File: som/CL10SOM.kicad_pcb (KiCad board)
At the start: 4 copper layers, 34.9 x 31.9 mm, 53 parts, among them IC1 10CL025YU256C8G, J1 Conn_01x02_Pin, U1 MT46H32M16LFBF-5 IT:C, U2 MX25L12833FM2, U6 AT93C46DN-SH-T, U7 SG3225CAN 50.0000M-TJGA6, X1 DF40C-120DS-0.4V51

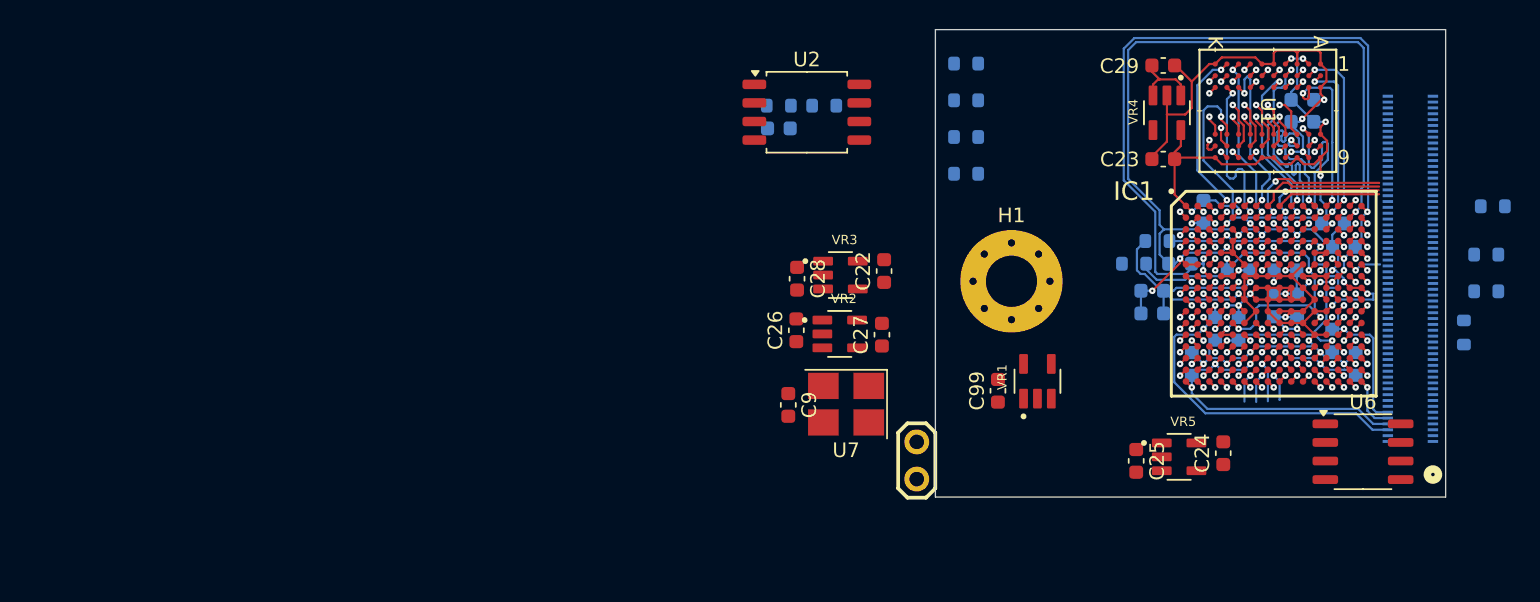
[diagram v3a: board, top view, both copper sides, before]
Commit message: Work in progress
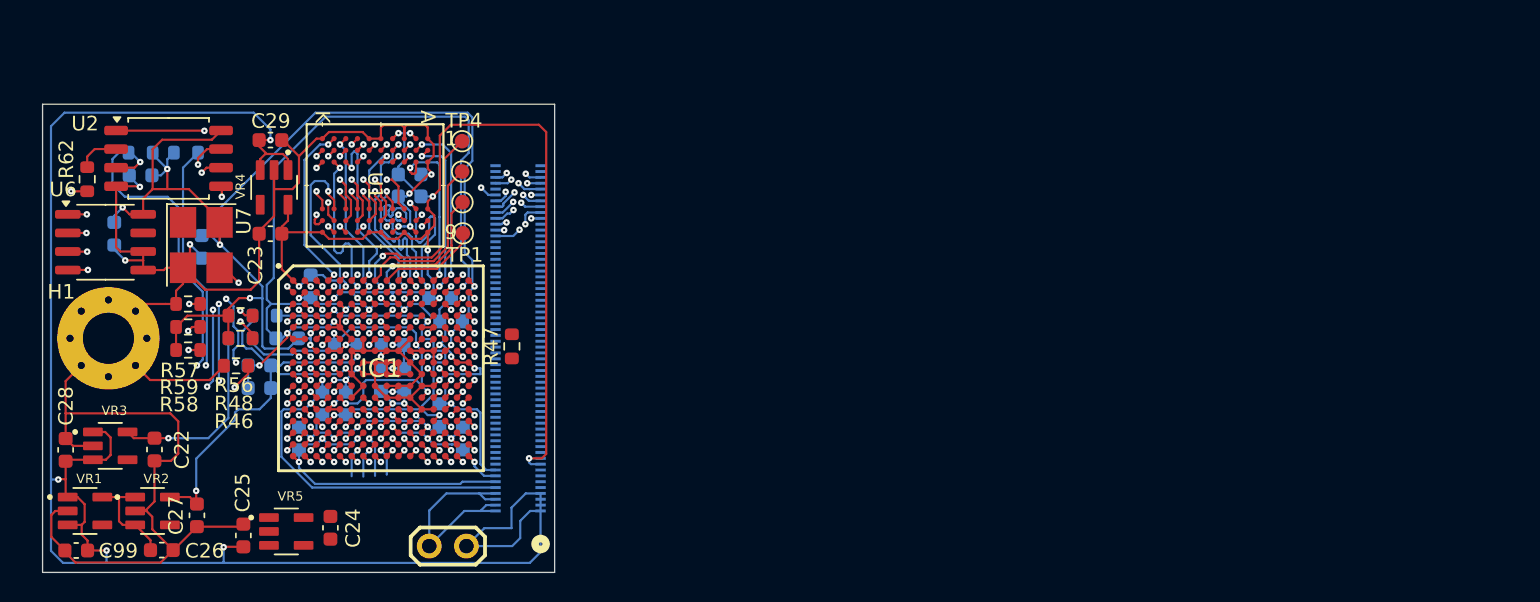
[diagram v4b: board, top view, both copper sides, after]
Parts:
- added C18: 100nF, Capacitor_SMD:C_0603_1608Metric, B.Cu at (88.7, 53.4)
- added TP1: TestPoint_Small, TestPoint:TestPoint_Pad_D1.0mm, F.Cu at (112.5, 53.3)
- added TP2: TestPoint_Small, TestPoint:TestPoint_Pad_D1.0mm, F.Cu at (112.5, 51.2)
- added TP3: TestPoint_Small, TestPoint:TestPoint_Pad_D1.0mm, F.Cu at (112.4, 49.1)
- added TP4: TestPoint_Small, TestPoint:TestPoint_Pad_D1.0mm, F.Cu at (112.4, 47.0)
- C9: moved to B.Cu
- R46, R47, R48, R56, R57, R58, R59, R62: moved to F.Cu
- moved U6 87.1 mm to (88.0, 53.9)
- moved R46 86.6 mm to (97.0, 62.4), turned to 0 degrees
- moved R48 85.3 mm to (97.3, 60.5), turned to 0 degrees
- moved R56 85.2 mm to (97.3, 59.0), turned to 0 degrees
- moved VR1 65.7 mm to (86.7, 72.3), turned to 0 degrees
- moved R47 65.1 mm to (115.8, 61.0)
- moved C99 63.9 mm to (86.0, 75.0), turned to 0 degrees
- moved H1 61.8 mm to (88.2, 60.5)
- moved R44 61.3 mm to (97.3, 60.5)
- moved C14 61.2 mm to (108.5, 63.4)
- moved C15 61.2 mm to (104.5, 61.0)
- moved C21 61.2 mm to (102.9, 65.0)
- moved C37 61.2 mm to (100.5, 60.5)
- moved C38 61.2 mm to (106.9, 63.4)
- moved C41 61.2 mm to (110.9, 65.8)
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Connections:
- IC1 pad B1: /B1-IO1 -> /EECS
- IC1 pad C2: /B1-IO2 -> /EECK
- IC1 pad D1: /B1-IO4 -> /EEDI
- IC1 pad E2: /B1-CLK0 -> /CLC50
- IC1 pad F3: /B1-IO3 -> /EEDO
- R49 pad 2: +3.3V -> +3V3
- R60 pad 2: +3.3V -> +3V3
- X1 pad 1: GND -> +5V
- X1 pad 10: VCCB4 -> VCCB2
- X1 pad 100: unconnected-(X1-Pad100) -> /B6-CLK5
- X1 pad 101: unconnected-(X1-Pad101) -> /B6-IO1
- X1 pad 102: unconnected-(X1-Pad102) -> /B6-IO7
- X1 pad 103: unconnected-(X1-Pad103) -> /B6-IO2
- X1 pad 104: unconnected-(X1-Pad104) -> /B6-IO8
- X1 pad 105: unconnected-(X1-Pad105) -> /B6-IO3
- X1 pad 106: unconnected-(X1-Pad106) -> /B6-IO9
- X1 pad 107: unconnected-(X1-Pad107) -> /B6-IO4
- X1 pad 108: unconnected-(X1-Pad108) -> /B6-IO10
- X1 pad 109: unconnected-(X1-Pad109) -> /B6-IO5
- X1 pad 110: unconnected-(X1-Pad110) -> /B6-IO11
- X1 pad 111: unconnected-(X1-Pad111) -> /B6-IO6
- X1 pad 113: unconnected-(X1-Pad113) -> /TMS
- X1 pad 114: unconnected-(X1-Pad114) -> /TDI
- X1 pad 115: unconnected-(X1-Pad115) -> /TDO
- X1 pad 116: unconnected-(X1-Pad116) -> /TCK
- X1 pad 12: VCCB5 -> VCCB3
- X1 pad 13: unconnected-(X1-Pad13) -> +2V5
- X1 pad 14: unconnected-(X1-Pad14) -> VCCB4
- X1 pad 15: unconnected-(X1-Pad15) -> +2V5
- X1 pad 16: unconnected-(X1-Pad16) -> VCCB5
- X1 pad 17: unconnected-(X1-Pad17) -> +1V8
- X1 pad 19: unconnected-(X1-Pad19) -> +1V8
- X1 pad 3: GND -> +5V
- X1 pad 41: /X1_41 -> unconnected-(X1-Pad41)
- X1 pad 42: /X1_42 -> unconnected-(X1-Pad42)
- X1 pad 43: /X1_43 -> unconnected-(X1-Pad43)
- X1 pad 44: /X1_44 -> unconnected-(X1-Pad44)
- X1 pad 45: /X1_45 -> unconnected-(X1-Pad45)
- X1 pad 46: /X1_46 -> unconnected-(X1-Pad46)
- X1 pad 47: /X1_47 -> unconnected-(X1-Pad47)
- X1 pad 48: /X1_48 -> unconnected-(X1-Pad48)
- X1 pad 49: /X1_49 -> unconnected-(X1-Pad49)
- X1 pad 5: unconnected-(X1-Pad5) -> +5V
- X1 pad 50: /X1_50 -> unconnected-(X1-Pad50)
- X1 pad 51: /X1_51 -> unconnected-(X1-Pad51)
- X1 pad 52: /X1_52 -> unconnected-(X1-Pad52)
- X1 pad 53: /X1_53 -> unconnected-(X1-Pad53)
- X1 pad 54: /X1_54 -> unconnected-(X1-Pad54)
- X1 pad 55: /X1_55 -> unconnected-(X1-Pad55)
- X1 pad 56: /X1_56 -> unconnected-(X1-Pad56)
- X1 pad 57: /X1_57 -> unconnected-(X1-Pad57)
- X1 pad 58: /X1_58 -> unconnected-(X1-Pad58)
- X1 pad 59: /X1_59 -> unconnected-(X1-Pad59)
- X1 pad 6: VCCB2 -> GND
- X1 pad 60: /X1_60 -> unconnected-(X1-Pad60)
- X1 pad 61: /X1_61 -> unconnected-(X1-Pad61)
- X1 pad 62: /X1_62 -> unconnected-(X1-Pad62)
- X1 pad 63: /X1_63 -> unconnected-(X1-Pad63)
- X1 pad 64: /X1_64 -> unconnected-(X1-Pad64)
- X1 pad 65: /X1_65 -> unconnected-(X1-Pad65)
- X1 pad 66: /X1_66 -> unconnected-(X1-Pad66)
- X1 pad 67: /X1_67 -> unconnected-(X1-Pad67)
- X1 pad 68: /X1_68 -> unconnected-(X1-Pad68)
- X1 pad 69: /X1_69 -> unconnected-(X1-Pad69)
- X1 pad 7: unconnected-(X1-Pad7) -> +5V
- X1 pad 70: /X1_70 -> unconnected-(X1-Pad70)
- X1 pad 71: /X1_71 -> unconnected-(X1-Pad71)
- X1 pad 72: /X1_72 -> unconnected-(X1-Pad72)
- X1 pad 73: /X1_73 -> unconnected-(X1-Pad73)
- X1 pad 74: /X1_74 -> unconnected-(X1-Pad74)
- X1 pad 75: /X1_75 -> unconnected-(X1-Pad75)
- X1 pad 76: /X1_76 -> unconnected-(X1-Pad76)
- X1 pad 77: /X1_77 -> unconnected-(X1-Pad77)
- X1 pad 78: /X1_78 -> unconnected-(X1-Pad78)
- X1 pad 79: /X1_79 -> unconnected-(X1-Pad79)
- X1 pad 8: VCCB3 -> GND
- X1 pad 80: /X1_80 -> unconnected-(X1-Pad80)
- X1 pad 9: unconnected-(X1-Pad9) -> +3.3V
- X1 pad 98: unconnected-(X1-Pad98) -> /B6-CLK4
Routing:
- net +5V: track 4.85 -> 123.2 mm, vias 0 -> 4
- net GND: track 182.7 -> 285.9 mm, vias 32 -> 35
- net /TDO: track 4.48 -> 56.4 mm, vias 1 -> 2
- net /TMS: track 9.17 -> 55.5 mm, vias 1 -> 3
- net /TDI: track 9.08 -> 53.5 mm, vias 1 -> 3
- net /TCK: track 8.43 -> 50.6 mm, vias 1 -> 3
- net +1V8: track 47.7 -> 85.1 mm, vias 9 -> 10
- net +3V3: track 58.3 -> 93.7 mm, vias 7 -> 11
- net /DATA0: track 2.93 -> 27.7 mm, vias 1 -> 4
- net /FL_D2: track 7.45 -> 31.6 mm, vias 1 -> 3
- net /nCSO: track 2.91 -> 22.9 mm, vias 1 -> 2
- net /DCLK: track 1.89 -> 21.8 mm, vias 1 -> 4
- net /EEDO: track 0.00 -> 19.8 mm, vias 0 -> 2
- net /FL_D3: track 6.44 -> 26.1 mm, vias 1 -> 3
- net /EECK: track 0.00 -> 19.4 mm, vias 0 -> 2
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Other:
- board size 34.9 x 31.9 mm -> 35 x 32 mm

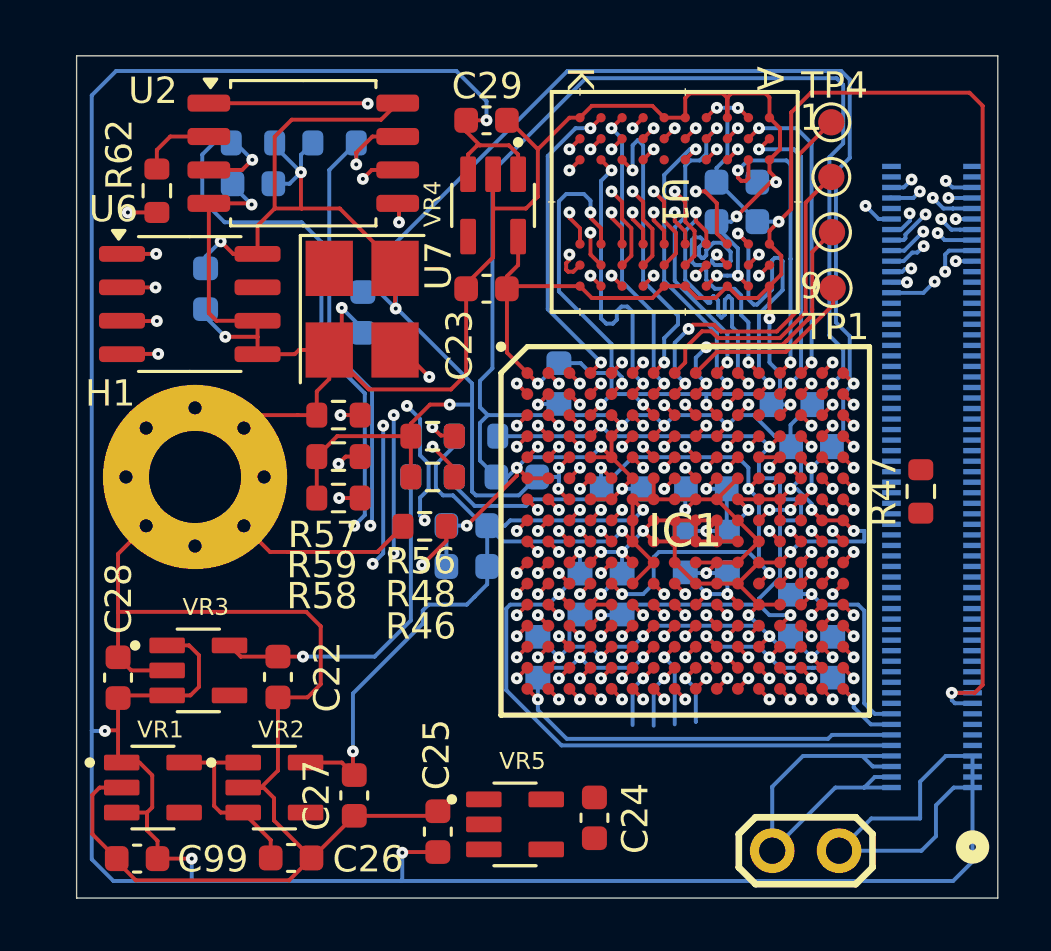
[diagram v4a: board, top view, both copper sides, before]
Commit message: Placement change
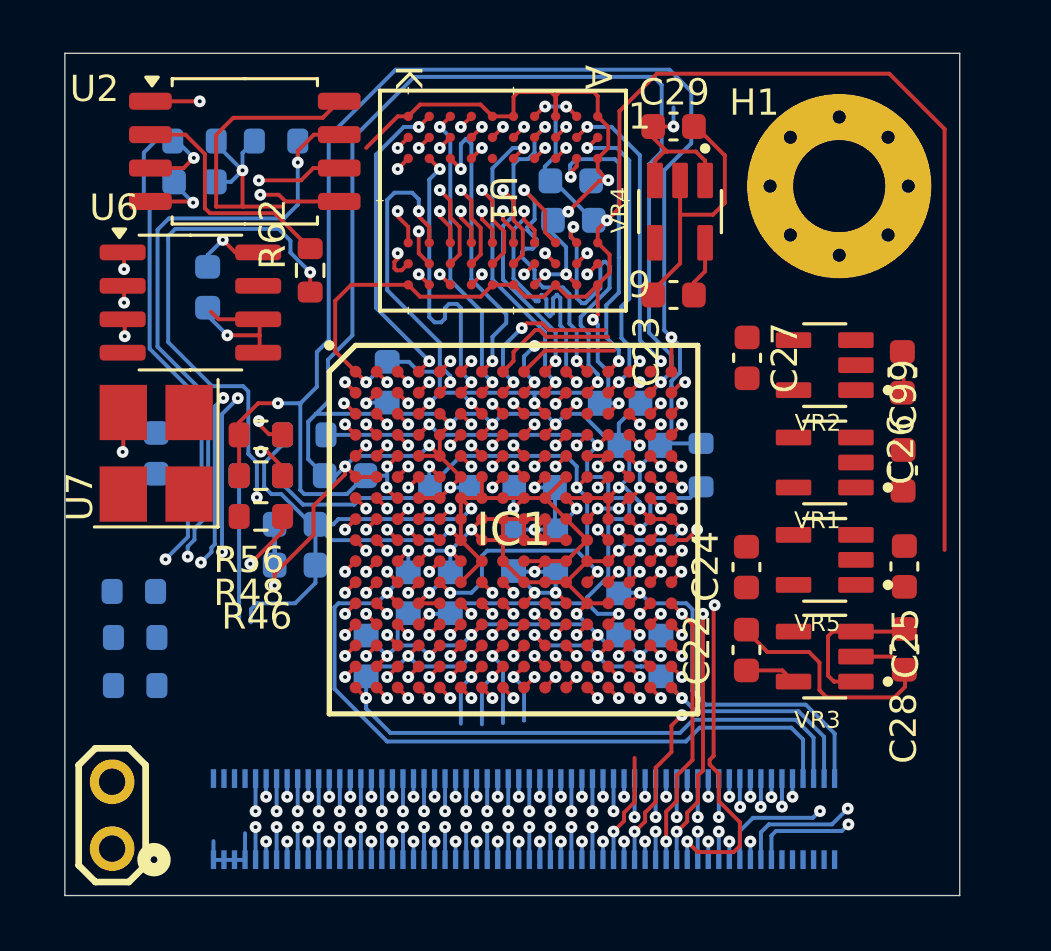
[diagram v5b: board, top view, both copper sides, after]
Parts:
- removed TP1, TP2, TP3, TP4: TestPoint_Small, TestPoint:TestPoint_Pad_D1.0mm
- R47, R57, R58, R59: moved to B.Cu
- moved C99 32.6 mm to (115.2, 60.2), turned to 90 degrees
- moved C28 29.9 mm to (115.2, 67.0), turned to 90 degrees
- moved C26 29.7 mm to (115.1, 56.5), turned to 90 degrees
- moved VR1 28.4 mm to (112.2, 60.0), turned to 180 degrees
- moved H1 26.9 mm to (112.7, 49.5)
- moved VR2 26.4 mm to (112.2, 56.2), turned to 180 degrees
- moved J1 25.2 mm to (85.1, 72.1), turned to -90 degrees
- moved VR3 23.8 mm to (112.2, 67.3), turned to 180 degrees
- moved C27 22.3 mm to (109.2, 56.0), turned to -90 degrees
- moved C25 20.4 mm to (115.2, 63.9), turned to 90 degrees
- moved X1 20.2 mm to (100.8, 73.5), turned to 0 degrees
- moved C22 17.8 mm to (109.2, 67.1), turned to -90 degrees
- moved VR5 15.5 mm to (112.2, 63.6), turned to 180 degrees
- moved C24 11.1 mm to (109.2, 63.9), turned to -90 degrees
- moved R58 10.5 mm to (86.0, 68.4)
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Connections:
- net /B2-IO1 renamed /B2-IO1p
- net /B2-IO13 renamed /B2-IO9p
- net /B2-IO14 renamed /B2-IO9n
- net /B2-IO2 renamed /B2-IO1n
- net /B2-IO3 renamed /B2-IO2p
- net /B2-IO5 renamed /B2-IO3p
- net /B2-IO9 renamed /B2-IO5n
- net /B3-IO1 renamed /B3-IO1p
- net /B3-IO13 renamed /B3-IO10p
- net /B3-IO18 renamed /B3-IO13p
- net /B3-IO19 renamed /B3-IO13n
- net /B3-IO2 renamed /B3-IO1n
- net /B3-IO4 renamed /B3-IO2n
- net /B3-IO6 renamed /B3-IO4-COp
- net /B4-IO10 renamed /B4-IO7p
- net /B4-IO14 renamed /B4-IO10p
- net /B4-IO15 renamed /B4-IO10n
- net /B4-IO17 renamed /B4-IO12-COp
- net /B4-IO18 renamed /B4-IO12-COn
- net /B4-IO2 renamed /B4-IO2p
- net /B4-IO3 renamed /B4-IO2n
- net /B4-IO4 renamed /B4-IO3p
- net /B4-IO7 renamed /B4-IO4n
- IC1 pad A12: /DDR_DQ4 -> /DDR_DQ3
- IC1 pad A14: /DDR_DQ13 -> /DDR_DQ12
- IC1 pad A15: /DDR_DQ12 -> /DDR_DQ13
- IC1 pad B11: /DDR_DQ3 -> /DDR_DQ4
- IC1 pad B16: /B6-IO6 -> /B6-IO4
- IC1 pad C15: /B6-IO11 -> /B6-IO8p
- IC1 pad C16: /B6-IO10 -> /B6-IO8n
- IC1 pad D15: /B6-IO9 -> /B6-IO7
- IC1 pad D16: /B6-IO8 -> /B6-IO6
- IC1 pad F13: /B6-IO3 -> /B6-IO2
- IC1 pad F14: /B6-IO7 -> /B6-IO5
- IC1 pad F15: /B6-IO5 -> /B6-IO3p
- IC1 pad F16: /B6-IO4 -> /B6-IO3n
- IC1 pad G15: /B6-IO2 -> /B6-IO1p
- IC1 pad G16: /B6-IO1 -> /B6-IO1n
- IC1 pad J13: /B5-IO16 -> /B5-IO11
- IC1 pad J14: /B5-IO15 -> /B5-IO10
- IC1 pad J15: /B5-IO14 -> /B5-IO9p
- IC1 pad J16: /B5-IO13 -> /B5-IO9n
- IC1 pad K1: /B2-IO4 -> /B2-IO2n
- IC1 pad K15: /B5-IO12 -> /B5-IO8p
- IC1 pad K16: /B5-IO11 -> /B5-IO8n
- IC1 pad K5: /B2-IO10 -> /B2-IO6
- IC1 pad L1: /B2-IO6 -> /B2-IO3n
- IC1 pad L13: /B5-IO8 -> /B5-IO6
- IC1 pad L14: /B5-IO7 -> /B5-IO5
- IC1 pad L15: /B5-IO10 -> /B5-IO7p
- IC1 pad L16: /B5-IO9 -> /B5-IO7n
- IC1 pad L3: /B2-IO7 -> /B2-IO4
- IC1 pad L4: /B2-IO11 -> /B2-IO7
- IC1 pad L7: /B3-IO17 -> /B3-IO12
- IC1 pad L8: /B3-IO20 -> /B3-IO14
- IC1 pad M10: /B4-IO12 -> /B4-IO8
- IC1 pad M6: /B3-IO10 -> /B3-IO7
- IC1 pad M7: /B3-IO12 -> /B3-IO9
- IC1 pad M8: /B3-IO21 -> /B3-IO15
- IC1 pad N11: /B4-IO13 -> /B4-IO9
- IC1 pad N12: /B4-IO16 -> /B4-IO11
- IC1 pad N15: /B5-IO6 -> /B5-IO4p
- IC1 pad N16: /B5-IO5 -> /B5-IO4n
- IC1 pad N2: /B2-IO8 -> /B2-IO5p
- IC1 pad N5: /B3-IO8 -> /B3-IO6p
- IC1 pad N6: /B3-IO9 -> /B3-IO6n
- IC1 pad N8: /B3-IO22 -> /B3-IO15
- IC1 pad P11: /B4-IO9 -> /B4-IO6
- IC1 pad P16: /B5-IO3 -> /B5-IO3n
- IC1 pad P6: /B3-IO11 -> /B3-IO8
- IC1 pad P8: /B3-IO23 -> /B3-IO16
- IC1 pad P9: /B4-IO8 -> /B4-IO5
- IC1 pad R1: /B2-IO12 -> /B2-IO8
- IC1 pad R12: /B4-IO6 -> /B4-IO4p
- IC1 pad R16: /B5-IO4 -> /B5-IO3p
- IC1 pad R3: /B3-IO3 -> /B3-IO2p
- IC1 pad R6: /B3-IO15 -> /B3-IO11p
- IC1 pad T11: /B4-IO5 -> /B4-IO3n
- IC1 pad T13: /B4-IO11 -> /B4-IO7n
- IC1 pad T2: /B3-IO5 -> /B3-IO3
- IC1 pad T4: /B3-IO7 -> /B3-IO5-COn
- IC1 pad T5: /B3-IO14 -> /B3-IO10n
- IC1 pad T6: /B3-IO16 -> /B3-IO11n
- X1 pad 10: VCCB2 -> /TCK
- X1 pad 100: /B6-CLK5 -> /B6-CLK4
- X1 pad 101: /B6-IO1 -> /B5-IO9p
- X1 pad 102: /B6-IO7 -> /B6-IO4
- X1 pad 103: /B6-IO2 -> /B5-IO9n
- X1 pad 104: /B6-IO8 -> /B6-IO5
- X1 pad 105: /B6-IO3 -> /B5-IO10
- X1 pad 106: /B6-IO9 -> /B6-IO6
- X1 pad 107: /B6-IO4 -> /B5-IO11
- X1 pad 108: /B6-IO10 -> /B6-IO7
- X1 pad 109: /B6-IO5 -> +3.3V
- X1 pad 11: +3.3V -> /TMS
- X1 pad 110: /B6-IO11 -> /B6-IO8n
- X1 pad 111: /B6-IO6 -> +3.3V
- X1 pad 112: unconnected-(X1-Pad112) -> /B6-IO8p
- X1 pad 113: /TMS -> +2V5
- X1 pad 114: /TDI -> VCCB2
- X1 pad 115: /TDO -> +2V5
- X1 pad 116: /TCK -> VCCB3
- X1 pad 117: unconnected-(X1-Pad117) -> +1V8
- X1 pad 118: unconnected-(X1-Pad118) -> VCCB4
- X1 pad 119: unconnected-(X1-Pad119) -> +1V8
- X1 pad 12: VCCB3 -> /TDI
- X1 pad 120: unconnected-(X1-Pad120) -> VCCB5
- X1 pad 13: +2V5 -> unconnected-(X1-Pad13)
- X1 pad 14: VCCB4 -> unconnected-(X1-Pad14)
- X1 pad 15: +2V5 -> unconnected-(X1-Pad15)
- X1 pad 16: VCCB5 -> unconnected-(X1-Pad16)
- X1 pad 17: +1V8 -> unconnected-(X1-Pad17)
- X1 pad 19: +1V8 -> unconnected-(X1-Pad19)
- X1 pad 80: unconnected-(X1-Pad80) -> /B5-IO1
- X1 pad 81: unconnected-(X1-Pad81) -> /B5-IO2
- X1 pad 82: unconnected-(X1-Pad82) -> /B5-IO4n
- X1 pad 83: unconnected-(X1-Pad83) -> /B5-IO3p
- X1 pad 84: unconnected-(X1-Pad84) -> /B5-IO4p
- X1 pad 85: unconnected-(X1-Pad85) -> /B5-IO3n
- X1 pad 86: unconnected-(X1-Pad86) -> /B5-IO5
- X1 pad 87: unconnected-(X1-Pad87) -> /B5-CLK7
- X1 pad 88: unconnected-(X1-Pad88) -> /B6-IO1p
- X1 pad 89: unconnected-(X1-Pad89) -> /B5-CLK6
- X1 pad 9: +3.3V -> /TDO
- X1 pad 90: unconnected-(X1-Pad90) -> /B6-IO1n
- X1 pad 91: unconnected-(X1-Pad91) -> /B5-IO6
- X1 pad 92: unconnected-(X1-Pad92) -> /B6-IO2
- X1 pad 93: unconnected-(X1-Pad93) -> /B5-IO7p
- X1 pad 94: unconnected-(X1-Pad94) -> /B6-IO3n
- X1 pad 95: unconnected-(X1-Pad95) -> /B5-IO7n
- X1 pad 96: unconnected-(X1-Pad96) -> /B6-IO3p
- X1 pad 97: unconnected-(X1-Pad97) -> /B5-IO8p
- X1 pad 98: /B6-CLK4 -> /B6-CLK5
- X1 pad 99: unconnected-(X1-Pad99) -> /B5-IO8n
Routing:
- net +5V: track 123.2 -> 14.8 mm, vias 4 -> 1
- net GND: track 285.9 -> 198.2 mm, vias 35 -> 34
- net /TDO: track 56.4 -> 8.32 mm
- net /TMS: track 55.5 -> 10.6 mm, vias 3 -> 2
- net /TDI: track 53.5 -> 10.5 mm, vias 3 -> 2
- net /TCK: track 50.6 -> 10.0 mm, vias 3 -> 2
- net /B5-IO11: track 1.52 -> 26.3 mm, vias 1 -> 2
- net /B6-IO8p: track 0.00 -> 22.2 mm, vias 0 -> 2
- net /B6-IO8n: track 0.00 -> 21.7 mm, vias 0 -> 2
- net /B5-IO10: track 2.32 -> 24.0 mm, vias 1 -> 2
- net /B5-IO9p: track 0.00 -> 21.2 mm, vias 0 -> 2
- net /B5-IO9n: track 0.00 -> 20.5 mm, vias 0 -> 2
- net /B5-IO8p: track 0.00 -> 19.7 mm, vias 0 -> 2
- net /B5-IO8n: track 0.00 -> 19.3 mm, vias 0 -> 2
- net /B5-IO7p: track 0.00 -> 18.7 mm, vias 0 -> 2
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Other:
- board size 35 x 32 mm -> 34 x 32 mm
